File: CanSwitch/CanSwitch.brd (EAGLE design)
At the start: 100 x 80 mm, 17 parts

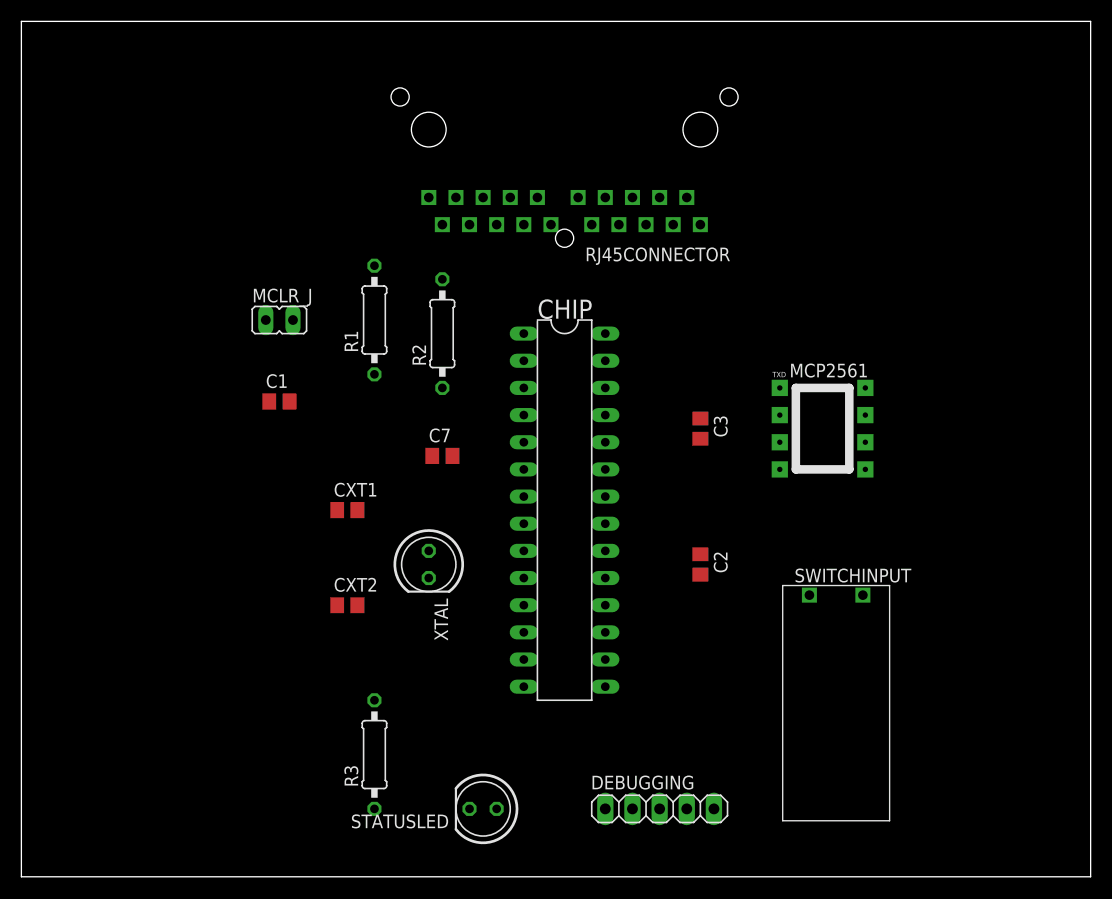
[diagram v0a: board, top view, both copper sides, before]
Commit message: first attempt to do proper wiring on the board
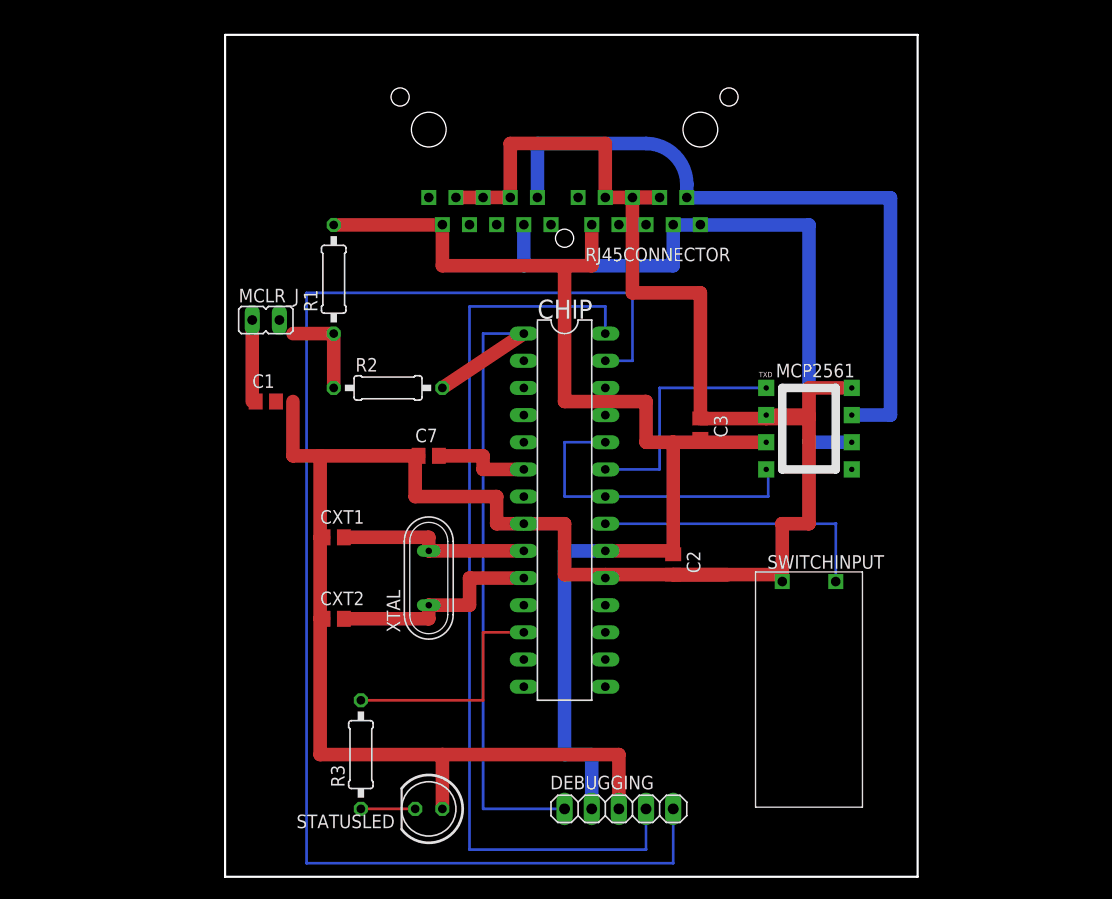
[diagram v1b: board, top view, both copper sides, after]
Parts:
- XTAL: value (none) -> 16MHz; device led:LED5MM -> special:QS
- moved R2 7.18 mm to (34.3, 45.7), turned to 0 degrees
- moved R1 5.39 mm to (29.2, 55.9)
- moved STATUSLED 5.08 mm to (38.1, 6.35)
- moved DEBUGGING 3.81 mm to (55.9, 6.35)
- moved SWITCHINPUT 2.84 mm to (73.7, 16.5)
- moved CXT1 2.84 mm to (29.2, 31.8)
- moved C2 2.54 mm to (61.0, 29.2)
- moved CXT2 1.80 mm to (29.2, 24.1)
- moved MCP2561 1.27 mm to (73.7, 41.9)
- moved R3 1.27 mm to (31.8, 11.4)
- moved C1 1.27 mm to (22.9, 44.5)
- moved MCLR_J 1.27 mm to (22.9, 52.1)
- moved XTAL 1.27 mm to (38.1, 27.9), turned to 90 degrees
- moved C7 1.27 mm to (38.1, 39.4)
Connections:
- removed net N$5: CHIP.10, CXT2.2, XTAL.K
- new net N$3: CHIP.10, CXT2.2, XTAL.1
- net N$6: now also XTAL.2; no longer XTAL.A
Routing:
- net GND: track 0.00 -> 232.2 mm
- net PGC: track 0.00 -> 132.1 mm
- net +5V: track 0.00 -> 115.0 mm
- net PGD: track 0.00 -> 86.4 mm
- net MCLR: track 0.00 -> 65.0 mm
- net CANH: track 0.00 -> 64.9 mm
- net CANL: track 0.00 -> 58.7 mm
- net RXD: track 0.00 -> 30.7 mm
- net INPUT: track 0.00 -> 27.0 mm
- net TXD: track 0.00 -> 22.7 mm
- net N$7: track 0.00 -> 21.6 mm
- net N$3: track 0.00 -> 20.6 mm
- net N$6: track 0.00 -> 18.1 mm
- net N$4: track 0.00 -> 9.21 mm
- net N$2: track 0.00 -> 8.89 mm
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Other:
- board size 100 x 80 mm -> 64.8 x 78.7 mm
